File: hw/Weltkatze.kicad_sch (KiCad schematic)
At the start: 0 parts

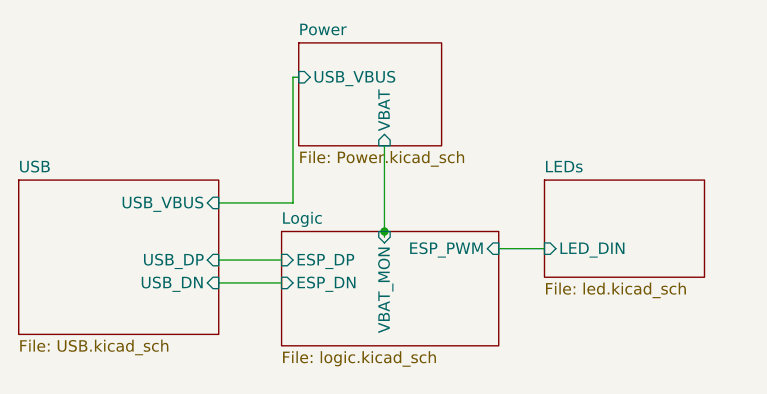
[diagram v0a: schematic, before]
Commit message: Rest of the owl
Finish major layout, minor tweaks can be made
E.g. rotating the LEDs so they look pretty

Still need to make it so the inner PCB is manufacturable
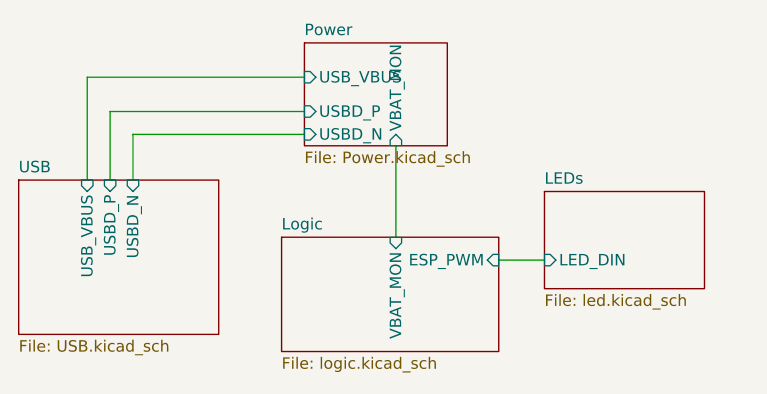
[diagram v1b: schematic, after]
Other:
- sheet Logic ports: added none; removed ESP_DN, ESP_DP
- sheet Power ports: added USBD_N, USBD_P, VBAT_MON; removed VBAT
- sheet USB ports: added USBD_N, USBD_P; removed USB_DN, USB_DP
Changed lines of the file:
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@@
 		(comment 1 "A light up Zigbee kitty")
 	)
-	(junction
-		(at 134.62 84.455)
-		(diameter 0)
-		(color 0 0 0 0)
-	)
-	(wire
-		(pts
-			(xy 116.205 90.17) (xy 123.19 90.17)
-		)
-		(stroke
-			(width 0)
-			(type default)
-		)
-	)
-	(wire
-		(pts
-			(xy 134.62 74.93) (xy 134.62 84.455)
-		)
-		(stroke
-			(width 0)
-			(type default)
-		)
-	)
-	(wire
-		(pts
-			(xy 116.205 81.28) (xy 124.46 81.28)
-		)
-		(stroke
-			(width 0)
-			(type default)
-		)
-	)
-	(wire
-		(pts
-			(xy 116.205 87.63) (xy 123.19 87.63)
-		)
-		(stroke
-			(width 0)
-			(type default)
-		)
-	)
-	(wire
-		(pts
-			(xy 134.62 84.455) (xy 134.62 85.09)
-		)
-		(stroke
-			(width 0)
-			(type default)
-		)
-	)
-	(wire
-		(pts
-			(xy 124.46 67.31) (xy 125.095 67.31)
-		)
-		(stroke
-			(width 0)
-			(type default)
-		)
-	)
-	(wire
-		(pts
-			(xy 147.32 86.36) (xy 152.4 86.36)
-		)
-		(stroke
-			(width 0)
-			(type default)
-		)
-	)
-	(wire
-		(pts
-			(xy 124.46 81.28) (xy 124.46 67.31)
+	(wire
+		(pts
+			(xy 104.14 78.74) (xy 104.14 71.12)
+		)
+		(stroke
+			(width 0)
+			(type default)
+		)
+	)
+	(wire
+		(pts
+			(xy 106.68 78.74) (xy 106.68 73.66)
+		)
+		(stroke
+			(width 0)
+			(type default)
+		)
+	)
+	(wire
+		(pts
+			(xy 106.68 73.66) (xy 125.73 73.66)
+		)
+		(stroke
+			(width 0)
+			(type default)
+		)
+	)
+	(wire
+		(pts
+			(xy 104.14 71.12) (xy 125.73 71.12)
+		)
+		(stroke
+			(width 0)
+			(type default)
+		)
+	)
+	(wire
+		(pts
+			(xy 101.6 67.31) (xy 125.73 67.31)
+		)
+		(stroke
+			(width 0)
+			(type default)
+		)
+	)
+	(wire
+		(pts
+			(xy 135.89 74.93) (xy 135.89 85.09)
+		)
+		(stroke
+			(width 0)
+			(type default)
+		)
+	)
+	(wire
+		(pts
+			(xy 147.32 87.63) (xy 152.4 87.63)
+		)
+		(stroke
+			(width 0)
+			(type default)
+		)
+	)
+	(wire
+		(pts
+			(xy 101.6 67.31) (xy 101.6 78.74)
 		)
 		(stroke
@@
 	)
 	(sheet
-		(at 123.19 84.455)
+		(at 123.19 85.09)
 		(size 24.13 12.7)
 		(fields_autoplaced yes)
@@
 		)
 		(property "Sheetname" "Logic"
-			(at 123.19 83.7434 0)
+			(at 123.19 84.3784 0)
 			(effects
 				(font
@@
 		)
 		(property "Sheetfile" "logic.kicad_sch"
-			(at 123.19 97.7396 0)
+			(at 123.19 98.3746 0)
 			(effects
 				(font
@@
 		)
 		(property "Field2" ""
-			(at 123.19 84.455 0)
+			(at 123.19 85.09 0)
 			(effects
 				(font
@@
 			)
 		)
-		(pin "ESP_DP" input
-			(at 123.19 87.63 180)
-			(effects
-				(font
-					(size 1.27 1.27)
-				)
-				(justify left)
-			)
-		)
 		(pin "ESP_PWM" input
-			(at 147.32 86.36 0)
-			(effects
-				(font
-					(size 1.27 1.27)
-				)
-				(justify right)
-			)
-		)
-		(pin "ESP_DN" input
-			(at 123.19 90.17 180)
-			(effects
-				(font
-					(size 1.27 1.27)
-				)
-				(justify left)
+			(at 147.32 87.63 0)
+			(effects
+				(font
+					(size 1.27 1.27)
+				)
+				(justify right)
 			)
 		)
 		(pin "VBAT_MON" input
-			(at 134.62 84.455 90)
+			(at 135.89 85.09 90)
 			(effects
 				(font
@@
 			)
 		)
-		(pin "USB_DP" input
-			(at 116.205 87.63 0)
-			(effects
-				(font
-					(size 1.27 1.27)
-				)
-				(justify right)
-			)
-		)
 		(pin "USB_VBUS" input
-			(at 116.205 81.28 0)
-			(effects
-				(font
-					(size 1.27 1.27)
-				)
-				(justify right)
-			)
-		)
-		(pin "USB_DN" input
-			(at 116.205 90.17 0)
+			(at 101.6 78.74 90)
+			(effects
+				(font
+					(size 1.27 1.27)
+				)
+				(justify right)
+			)
+		)
+		(pin "USBD_N" input
+			(at 106.68 78.74 90)
+			(effects
+				(font
+					(size 1.27 1.27)
+				)
+				(justify right)
+			)
+		)
+		(pin "USBD_P" input
+			(at 104.14 78.74 90)
 			(effects
 				(font
@@
 	)
 	(sheet
-		(at 152.4 78.74)
+		(at 152.4 80.01)
 		(size 17.78 10.795)
 		(fields_autoplaced yes)
@@
 		)
 		(property "Sheetname" "LEDs"
-			(at 152.4 78.0284 0)
+			(at 152.4 79.2984 0)
 			(effects
 				(font
@@
 		)
 		(property "Sheetfile" "led.kicad_sch"
-			(at 152.4 90.1196 0)
+			(at 152.4 91.3896 0)
 			(effects
 				(font
@@
 		)
 		(pin "LED_DIN" input
-			(at 152.4 86.36 180)
+			(at 152.4 87.63 180)
 			(effects
 				(font
@@
 	)
 	(sheet
-		(at 125.095 63.5)
+		(at 125.73 63.5)
 		(size 15.875 11.43)
 		(fields_autoplaced yes)
@@
 		)
 		(property "Sheetname" "Power"
-			(at 125.095 62.7884 0)
+			(at 125.73 62.7884 0)
 			(effects
 				(font
@@
 		)
 		(property "Sheetfile" "Power.kicad_sch"
-			(at 125.095 75.5146 0)
+			(at 125.73 75.5146 0)
 			(effects
 				(font
@@
 		)
 		(pin "USB_VBUS" input
-			(at 125.095 67.31 180)
+			(at 125.73 67.31 180)
 			(effects
 				(font
@@
 			)
 		)
-		(pin "VBAT" input
-			(at 134.62 74.93 270)
-			(effects
-				(font
+		(pin "VBAT_MON" input
+			(at 135.89 74.93 270)
+			(effects
+				(font
+					(size 1.27 1.27)
+				)
+				(justify left)
+			)
+		)
+		(pin "USBD_N" input
+			(at 125.73 73.66 180)
+			(effects
+				(font
+					(size 1.27 1.27)
+				)
+				(justify left)
+			)
+		)
+		(pin "USBD_P" input
+			(at 125.73 71.12 180)
+			(effects
+				(font
